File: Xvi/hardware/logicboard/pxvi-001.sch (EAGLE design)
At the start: 72 parts, among them J1 MKR, J4 QWIIC_RIGHT_ANGLE, J5 SPI, J6 QWIIC_RIGHT_ANGLE, J7 DIN5, K1 G5V1, Q1 60V/32A/35mΩ, Q10 60V/32A/35mΩ, Q11 60V/32A/35mΩ, Q12 60V/32A/35mΩ, Q13 60V/32A/35mΩ, Q14 60V/32A/35mΩ, Q15 60V/32A/35mΩ, Q16 60V/32A/35mΩ, Q2 60V/32A/35mΩ, Q3 60V/32A/35mΩ, Q4 60V/32A/35mΩ, Q5 60V/32A/35mΩ, Q6 60V/32A/35mΩ, Q7 60V/32A/35mΩ, Q8 60V/32A/35mΩ, Q9 60V/32A/35mΩ, T1 2SC1815, U1 DS18B20, X1 ADAFRUIT-PCA9685, X2 MKDSN1,5/2-5,08

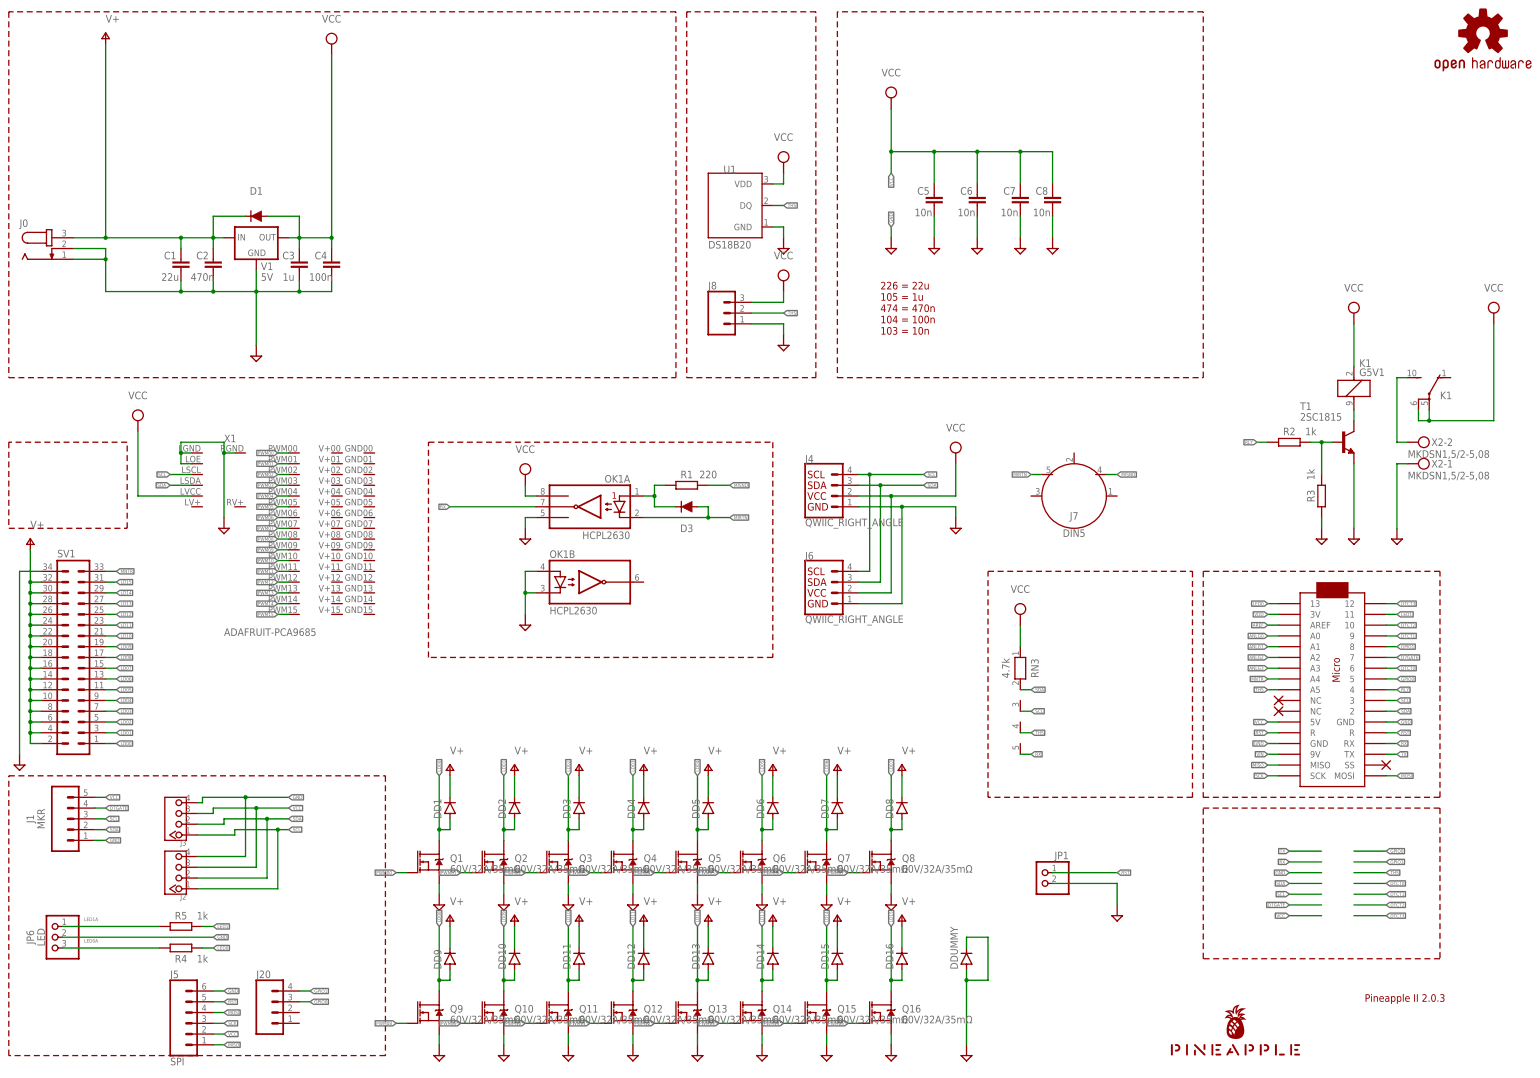
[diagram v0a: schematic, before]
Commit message: Cap and diode.
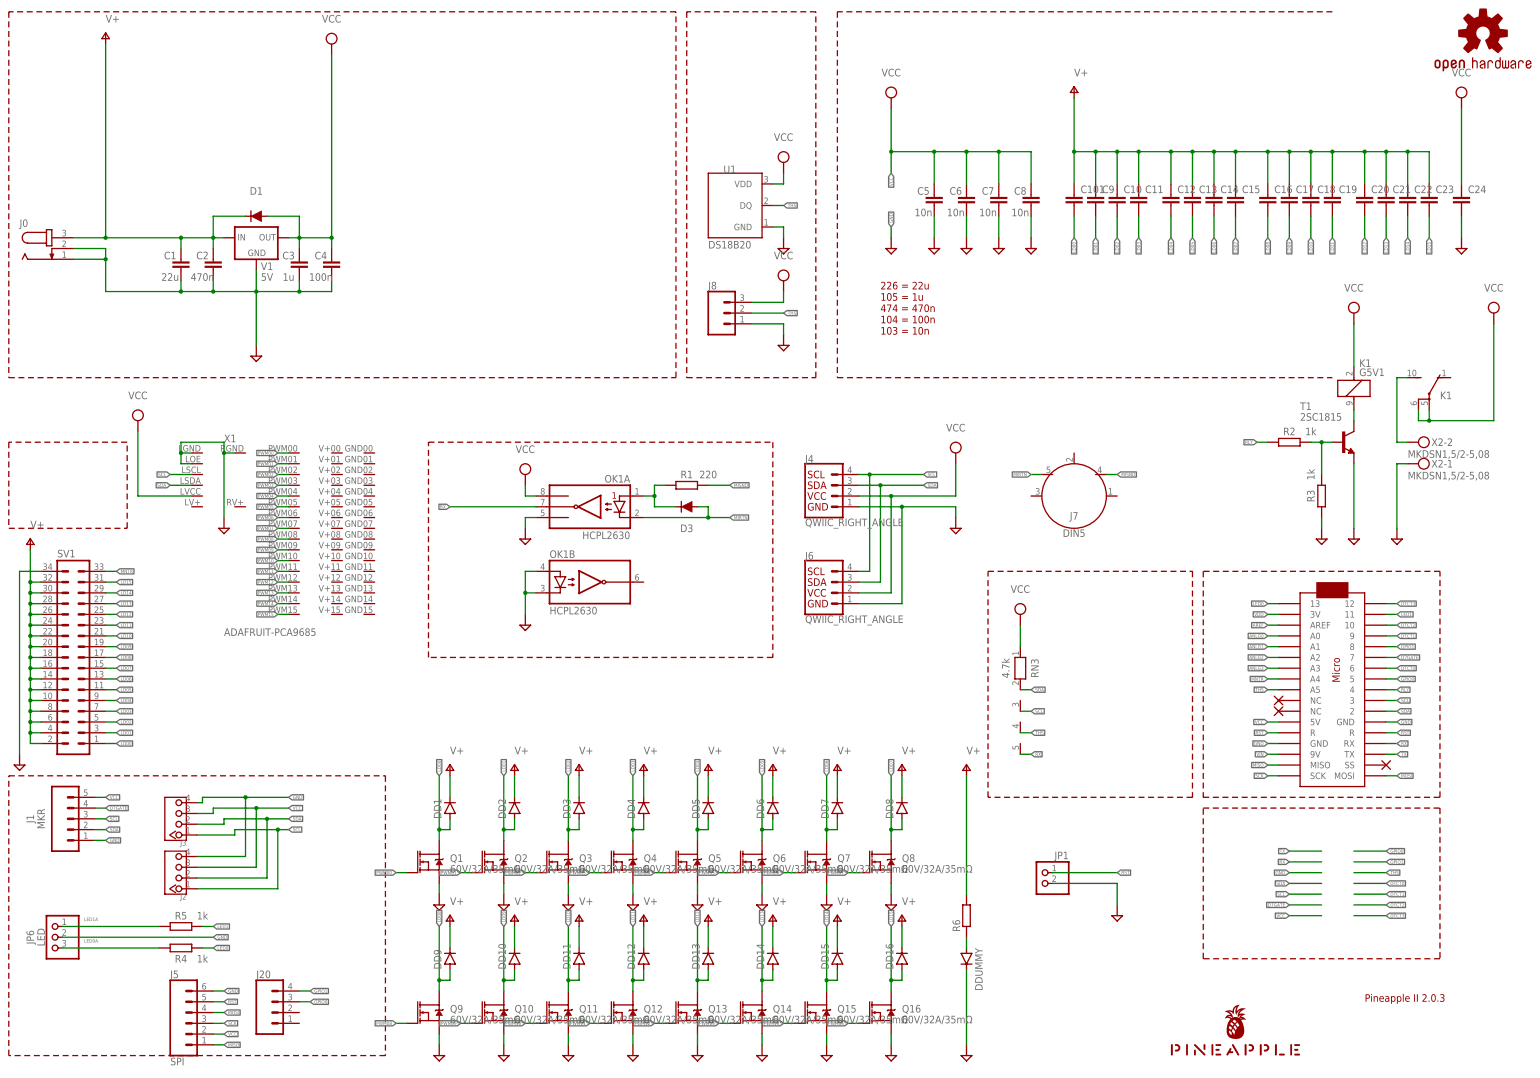
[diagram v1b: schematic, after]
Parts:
- added C10, C101, C11, C12, C13, C14, C15, C16, C17, C18, C19, C20, C21, C22, C23, C24, C9: (no value), rcl:C-EUC3216
- added R6: (no value), rcl:R-EU_R3216
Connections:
- new net N$3: DDUMMY.A, R6.1
- net GND: now also C24.2; no longer DDUMMY.A
- net LD00: now also C101.2
- net LD01: now also C9.2
- net LD02: now also C10.2
- net LD03: now also C11.2
- net LD04: now also C12.2
- net LD05: now also C13.2
- net LD06: now also C14.2
- net LD07: now also C15.2
- net LD08: now also C16.2
- net LD09: now also C17.2
- net LD10: now also C18.2
- net LD11: now also C19.2
- net LD12: now also C20.2
- net LD13: now also C21.2
- net LD14: now also C22.2
- net LD15: now also C23.2
- net V+: now also C10.1, C101.1, C11.1, C12.1, C13.1, C14.1, C15.1, C16.1, C17.1, C18.1, C19.1, C20.1, C21.1, C22.1, C23.1, C9.1, R6.2
- net VCC: now also C24.1
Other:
- moved on the sheet: C6, C7, C8, DDUMMY
